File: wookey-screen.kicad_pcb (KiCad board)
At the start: 4 copper layers, 43 x 66 mm, 21 parts, among them P8001 ER-CON50HT-1, P8002 CPU, U8001 ADS7846

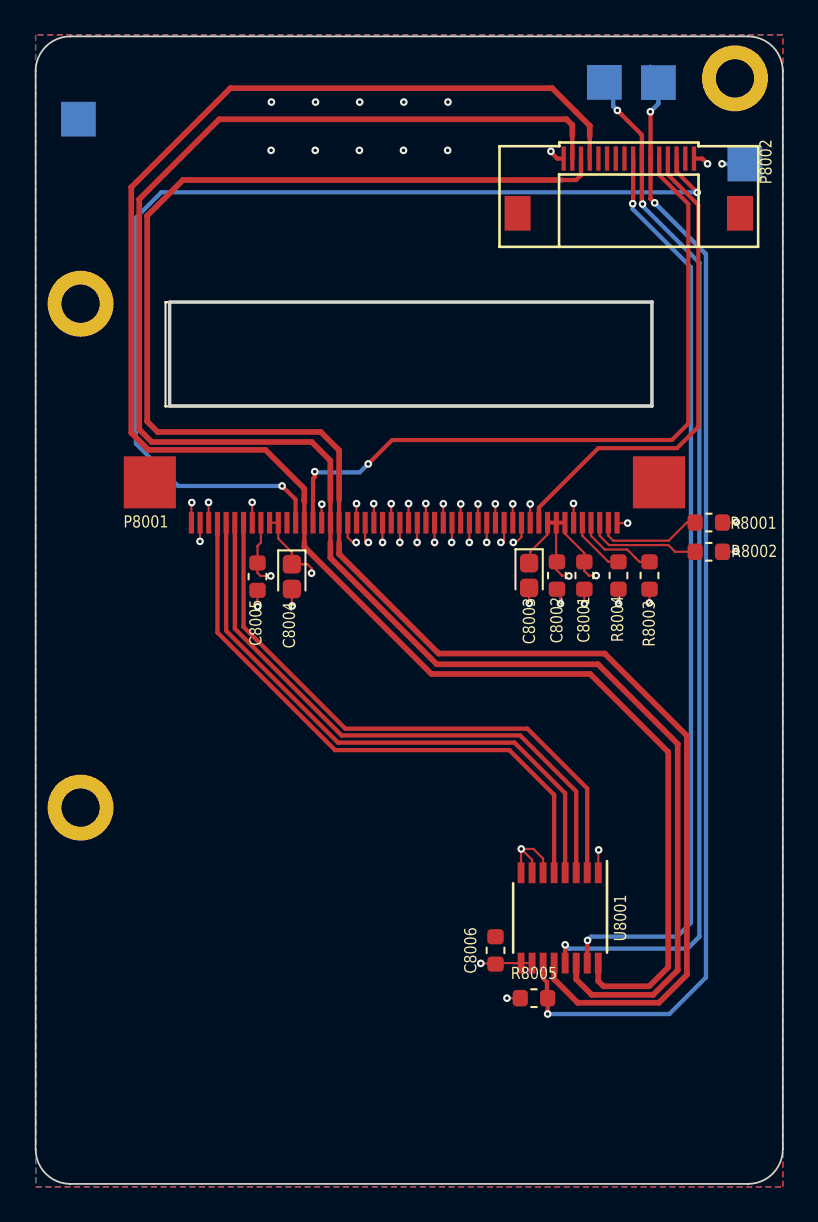
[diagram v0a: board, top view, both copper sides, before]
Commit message: [enhancement] global cleanup
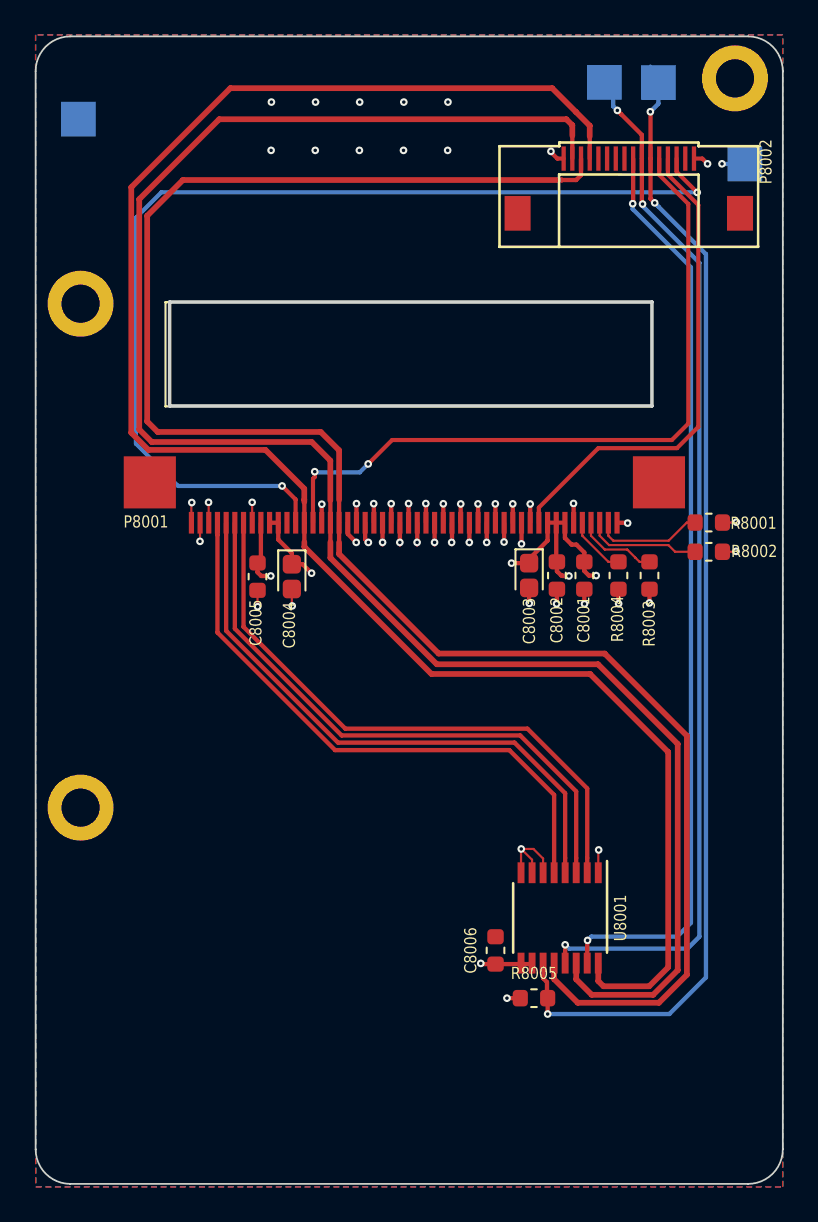
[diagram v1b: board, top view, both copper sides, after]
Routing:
- net GND: track 48.4 -> 75.2 mm
- net +3V3: track 30.3 -> 40.2 mm, vias 11 -> 12
